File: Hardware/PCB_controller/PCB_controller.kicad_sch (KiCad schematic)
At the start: 19 parts, among them J1 Conn_01x02, J2 Conn_01x06, J3 Conn_01x04, J4 Conn_ST_STDC14, SW1 SW_SPDT, U1 STM32G431KBTx, U2 AZ1117-3.3

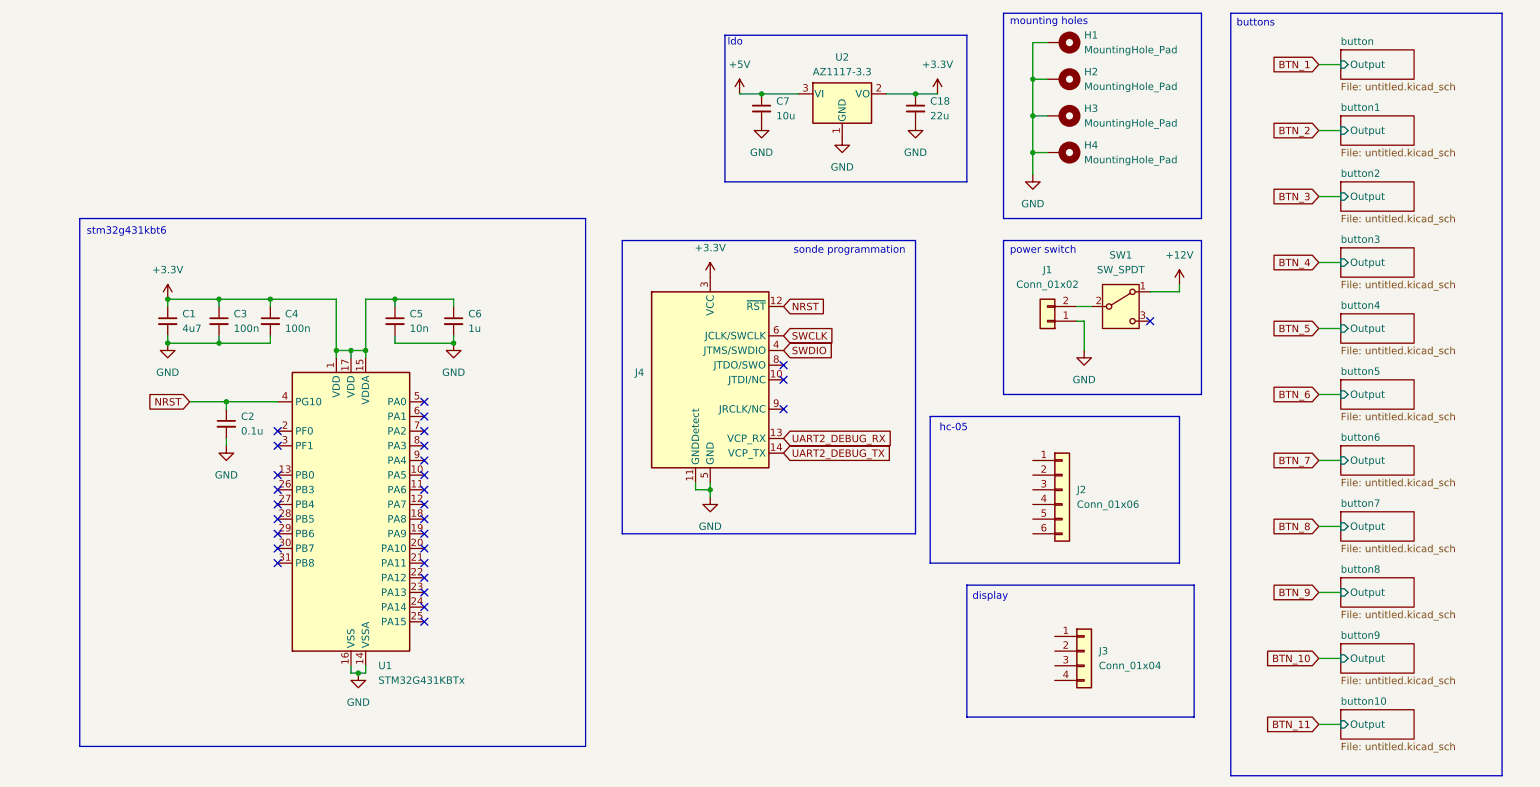
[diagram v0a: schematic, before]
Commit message: finished controller pcb
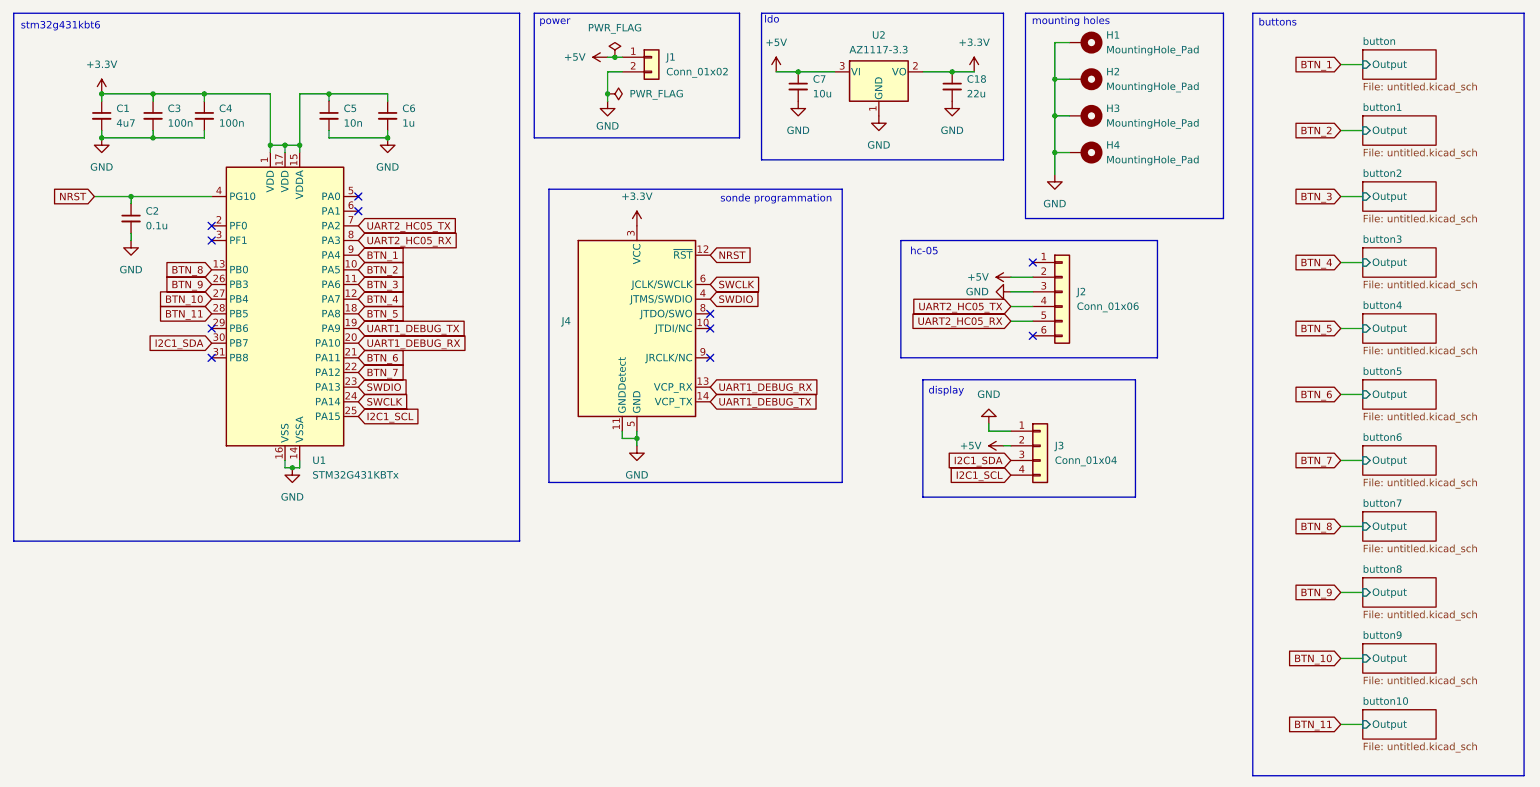
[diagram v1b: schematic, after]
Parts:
- removed SW1: SW_SPDT, mylib:472123010111, symbol Switch:SW_SPDT
- J1: footprint Connector_AMASS:AMASS_XT60-M_1x02_P7.20mm_Vertical -> (none)
- J2: footprint (none) -> Connector_JST:JST_EH_B6B-EH-A_1x06_P2.50mm_Vertical
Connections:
- net UART2_DEBUG_RX is gone; now on net UART1_DEBUG_RX: J4.13 (VCP_RX)
- net UART2_DEBUG_TX is gone; now on net UART1_DEBUG_TX: J4.14 (VCP_TX)
- net +5V: now also J1.1 (Pin_1), J2.2 (Pin_2), J3.2 (Pin_2)
- net BTN_1: now also U1.9 (PA4)
- net BTN_10: now also U1.27 (PB4)
- net BTN_11: now also U1.28 (PB5)
- net BTN_2: now also U1.10 (PA5)
- net BTN_3: now also U1.11 (PA6)
- net BTN_4: now also U1.12 (PA7)
- net BTN_5: now also U1.18 (PA8)
- net BTN_6: now also U1.21 (PA11)
- net BTN_7: now also U1.22 (PA12)
- net BTN_8: now also U1.13 (PB0)
- net BTN_9: now also U1.26 (PB3)
- net GND: now also J1.2 (Pin_2), J2.3 (Pin_3), J3.1 (Pin_1); no longer J1.1 (Pin_1)
- net SWCLK: now also U1.24 (PA14)
- net SWDIO: now also U1.23 (PA13)
- net I2C1_SDA: now reaches J3.3 (Pin_3)
- net I2C1_SDA: now also U1.30 (PB7)
- net I2C1_SCL: now reaches J3.4 (Pin_4)
- net I2C1_SCL: now also U1.25 (PA15)
- net UART1_DEBUG_TX: now reaches U1.19 (PA9)
- net UART1_DEBUG_RX: now reaches U1.20 (PA10)
- net UART2_HC05_TX: now reaches U1.7 (PA2)
- net UART2_HC05_TX: now also J2.4 (Pin_4)
- net UART2_HC05_RX: now reaches U1.8 (PA3)
- net UART2_HC05_RX: now also J2.5 (Pin_5)
- no-connect marks 29 -> 11
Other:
- note added: "power"
- note removed: "power switch"
- moved on the sheet: C1, C18, C2, C3, C4, C5, C6, C7, H1, H2, H3, H4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

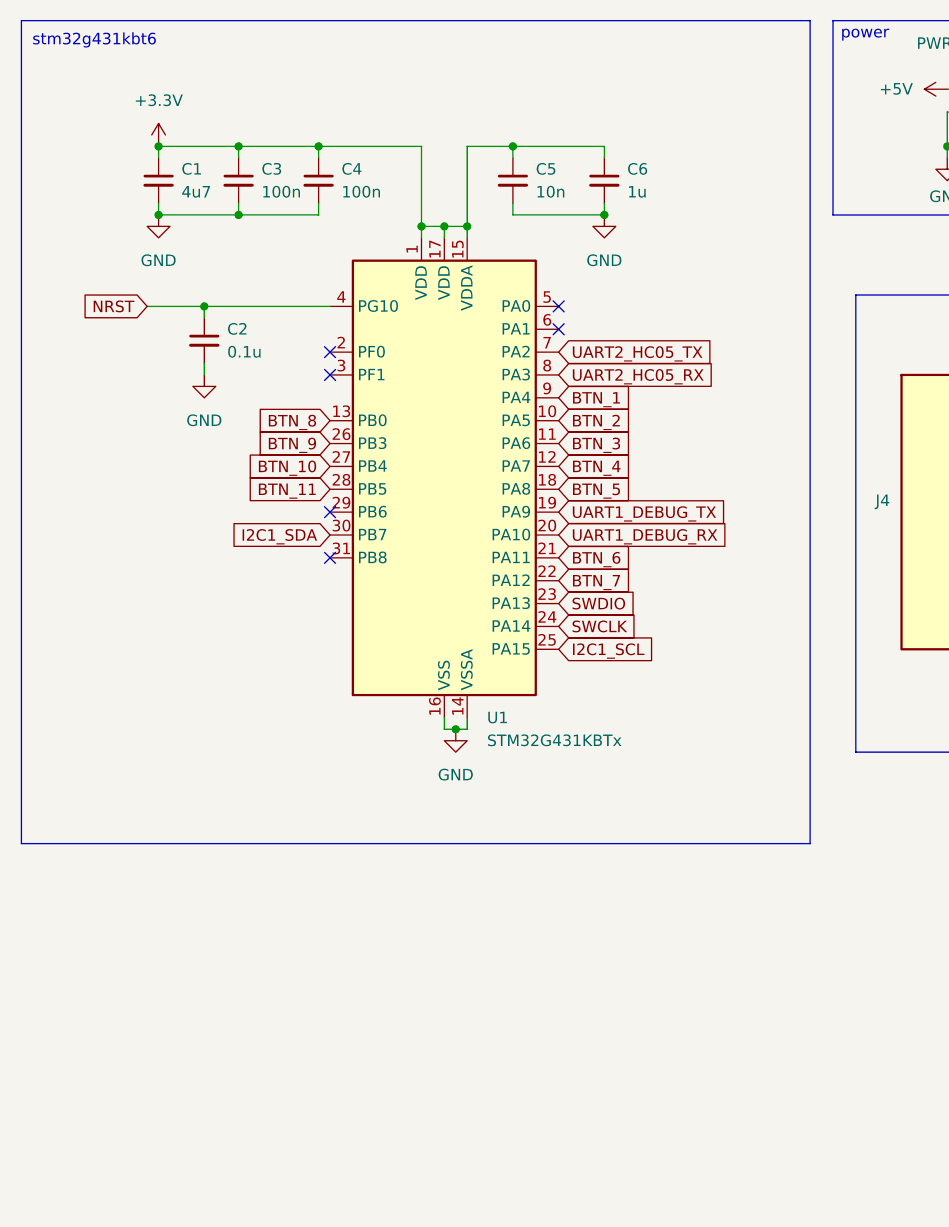
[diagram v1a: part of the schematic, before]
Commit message: started controller PCB
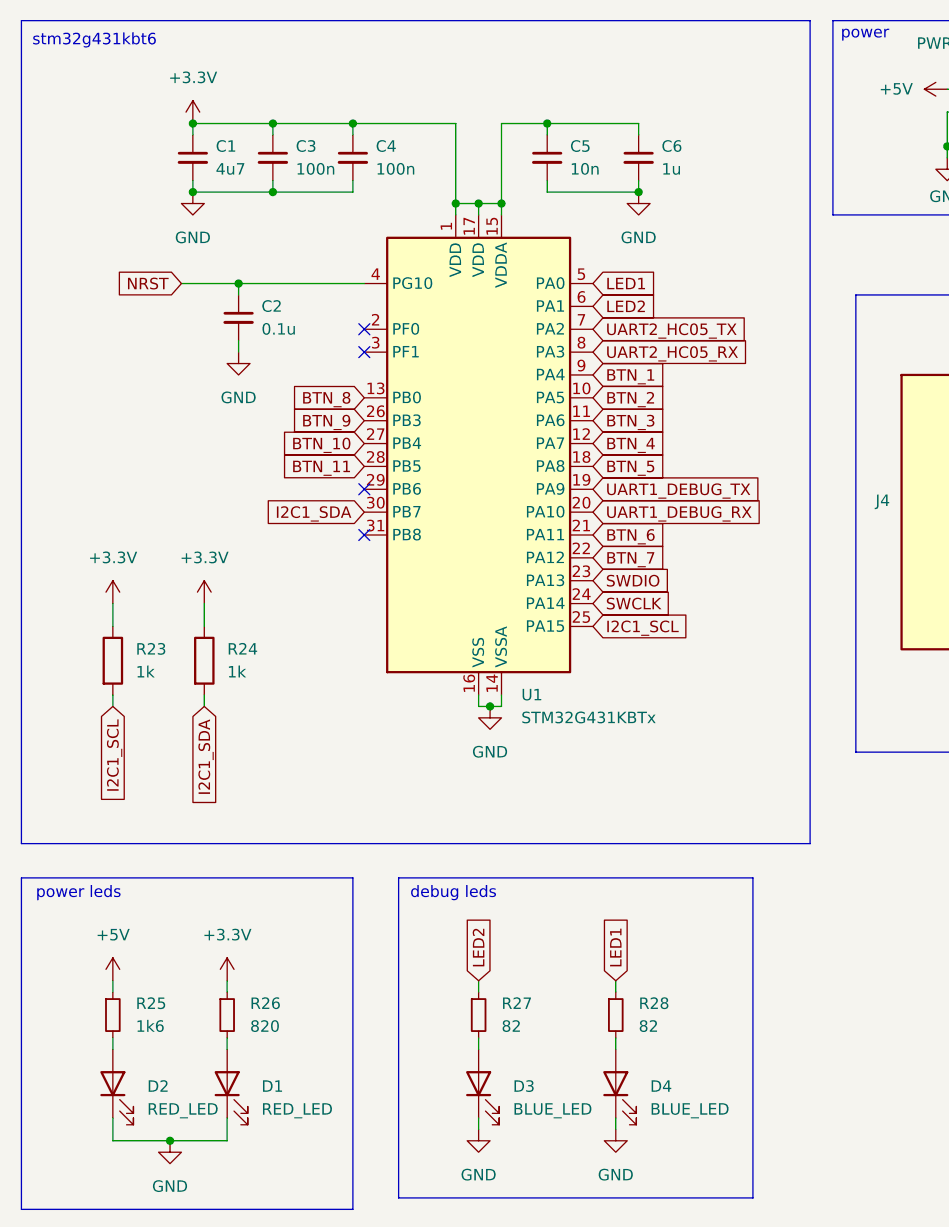
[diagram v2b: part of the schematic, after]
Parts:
- added D1, D2: RED_LED, LED_SMD:LED_0603_1608Metric, symbol Device:LED
- added D3, D4: BLUE_LED, LED_SMD:LED_0603_1608Metric, symbol Device:LED
- added R23, R24: 1k, Resistor_SMD:R_0402_1005Metric_Pad0.72x0.64mm_HandSolder, symbol Device:R
- added R25: 1k6, Resistor_SMD:R_0402_1005Metric_Pad0.72x0.64mm_HandSolder, symbol Device:R_Small
- added R26: 820, Resistor_SMD:R_0402_1005Metric_Pad0.72x0.64mm_HandSolder, symbol Device:R_Small
- added R27, R28: 82, Resistor_SMD:R_0402_1005Metric_Pad0.72x0.64mm_HandSolder, symbol Device:R_Small
- C1, C6, C7: footprint Capacitor_SMD:C_0402_1005Metric -> Capacitor_SMD:C_0603_1608Metric
- C2, C3, C4, C5: footprint Capacitor_SMD:C_0402_1005Metric -> Capacitor_SMD:C_0402_1005Metric_Pad0.74x0.62mm_HandSolder
- H1, H2, H3, H4: footprint (none) -> MountingHole:MountingHole_3.2mm_M3_Pad_Via
- J1: footprint (none) -> Connector_JST:JST_EH_B2B-EH-A_1x02_P2.50mm_Vertical
- J3: footprint (none) -> Connector_JST:JST_EH_B4B-EH-A_1x04_P2.50mm_Vertical
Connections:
- net +3.3V: now also R23.1, R24.1, R26.1
- net +5V: now also R25.1
- net GND: now also D1.1 (K), D2.1 (K), D3.1 (K), D4.1 (K)
- net I2C1_SCL: now also R23.2
- net I2C1_SDA: now also R24.2
- net LED1: now reaches U1.5 (PA0)
- net LED1: now also R28.1
- net LED2: now reaches U1.6 (PA1)
- net LED2: now also R27.1
- new net: D4.2 (A), R28.2
- new net: D1.2 (A), R26.2
- new net: D3.2 (A), R27.2
- new net: D2.2 (A), R25.2
- no-connect marks 11 -> 9
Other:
- note added: "debug leds"
- note added: "power leds"
- moved on the sheet: C1, C2, C3, C4, C5, C6, U1
